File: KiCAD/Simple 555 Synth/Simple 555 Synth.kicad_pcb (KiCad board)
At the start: 2 copper layers, 10 parts, among them P1 PWR_5v, P4 EasyLAB_LOGO, U1 555-timer, U2 555-timer

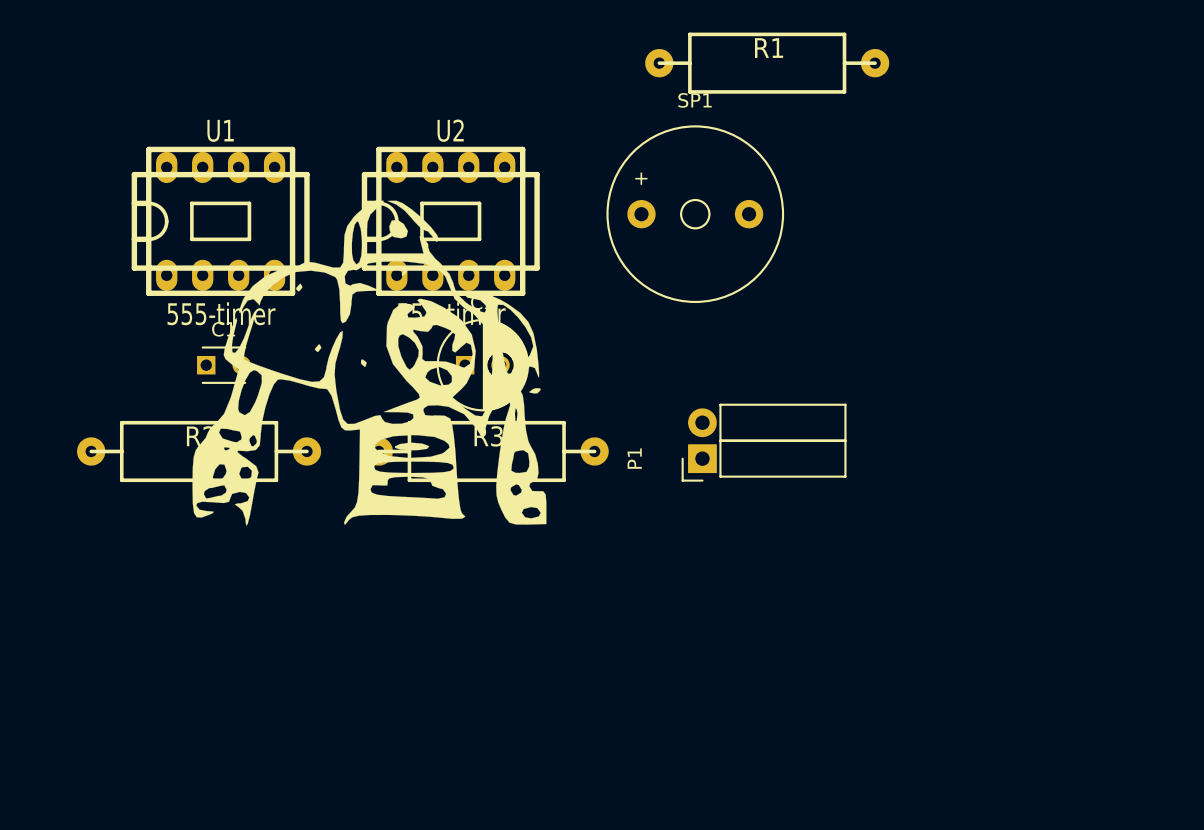
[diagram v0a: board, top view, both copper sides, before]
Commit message: schema en printplaat Versie 20180625 0.6
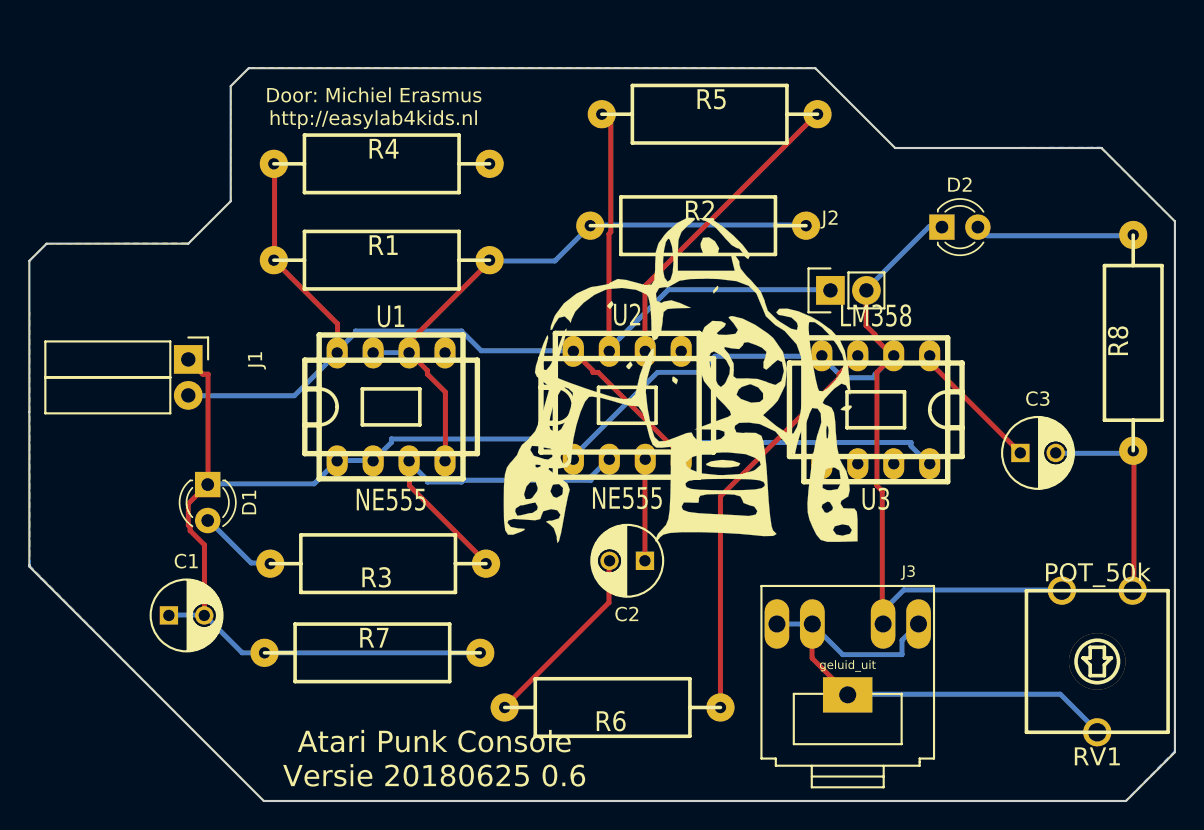
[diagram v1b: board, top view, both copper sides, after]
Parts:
- removed P1: PWR_5v, Socket_Strips:Socket_Strip_Angled_1x02
- removed SP1: Luidspreker, Buzzers_Beepers:Buzzer_12x9.5RM7.6
- added C2: 10uF, Capacitors_ThroughHole:C_Radial_D5_L11_P2.5, F.Cu at (66.5, 53.4)
- added D1: LED1, LEDs:LED_D3.0mm, F.Cu at (35.7, 48.1)
- added D2: LED2, LEDs:LED_D3.0mm, F.Cu at (87.5, 29.9)
- added J1: Stroom, Socket_Strips:Socket_Strip_Angled_1x02, F.Cu at (34.3, 39.2)
- added J2: CapacitorInput, Socket_Strips:Socket_Strip_Straight_1x02, F.Cu at (79.7, 34.3)
- added J3: geluid_uit, footprints:Tayda_3.5mm_stereo_TRS_jack_A-853, F.Cu at (80.9, 61.3)
- added R4: R470K, w_pth_resistors:RC07, F.Cu at (48.0, 25.4)
- added R5: R_PHOTO2, w_pth_resistors:RC07, F.Cu at (71.1, 21.9)
- added R6: R1K, w_pth_resistors:RC07, F.Cu at (64.3, 63.8)
- added R7: R1K, w_pth_resistors:RC07, F.Cu at (47.3, 59.9)
- added R8: R1k, w_pth_resistors:RC07, F.Cu at (101.0, 38.0)
- added RV1: POT_50k, w_pth_resistors:trimmer_ecp_ca9-v10, F.Cu at (98.5, 60.6)
- added U3: LM358, w_pth_circuits:dil_8-300_socket, F.Cu at (82.9, 42.8)
- C1: value 01.uF -> 0.1uF; footprint Capacitors_ThroughHole:C_Disc_D3_P2.5 -> Capacitors_ThroughHole:C_Radial_D5_L11_P2.5
- C3: footprint Capacitors_ThroughHole:C_Radial_D6.3_L11.2_P2.5 -> Capacitors_ThroughHole:C_Radial_D5_L11_P2.5
- R1: value R100k -> R470K
- R2: value R1k -> R_PHOTO1
- R3: value R50k -> R1K
- U1, U2: value 555-timer -> NE555
- moved C3 39.7 mm to (93.1, 45.8)
- moved R2 38.7 mm to (70.3, 29.8)
- moved R1 30.6 mm to (48.0, 32.2)
- moved P4 22.0 mm to (69.1, 40.4)
- moved U2 18.0 mm to (65.3, 42.5)
- moved C1 17.9 mm to (32.9, 57.3)
- moved U1 17.8 mm to (48.6, 42.6)
- moved R3 11.0 mm to (47.7, 53.6), turned to 180 degrees
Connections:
- C1 pad 1: /TRG -> /TRG1
- C1 pad 2: /DIS -> /TRG1
- C3 pad 1: /SPKR -> Net-(C3-Pad1)
- R1 pad 1: /DIS2 -> /RST2
- R1 pad 2: /VSS -> /RST1
- R2 pad 1: /THR -> /RST1
- R2 pad 2: /DIS -> /RST1
- R3 pad 1: /DIS -> /geluid1
- R3 pad 2: /VSS -> Net-(D1-Pad2)
- U1 pad 1: /VSS -> /TRG1
- U1 pad 2: /TRG -> /TRG1
- U1 pad 3: /OUT -> /geluid1
- U1 pad 4: /OUT -> /RST1
- U1 pad 6: /THR -> /RST1
- U1 pad 7: /DIS -> /RST1
- U1 pad 8: /RESET2 -> /RST2
- U2 pad 1: /VSS -> /TRG1
- U2 pad 2: /OUT -> /geluid1
- U2 pad 3: /SPKR -> Net-(C2-Pad1)
- U2 pad 4: /RESET2 -> /RST2
- U2 pad 6: /DIS2 -> Net-(R5-Pad2)
- U2 pad 7: /DIS2 -> /Cap+
- U2 pad 8: /RESET2 -> /RST2
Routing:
- net /TRG1: track 0.00 -> 145.5 mm
- net /RST2: track 0.00 -> 75.2 mm
- net /RST1: track 0.00 -> 43.8 mm
- net Net-(J3-Pad1): track 0.00 -> 37.5 mm
- net /Cap+: track 0.00 -> 34.8 mm
- net Net-(R6-Pad1): track 0.00 -> 28.9 mm
- net /geluid1: track 0.00 -> 25.3 mm
- net Net-(R5-Pad2): track 0.00 -> 21.9 mm
- net Net-(C3-Pad2): track 0.00 -> 15.7 mm
- net Net-(C2-Pad2): track 0.00 -> 13.4 mm
- net Net-(D2-Pad2): track 0.00 -> 11.3 mm
- net Net-(C3-Pad1): track 0.00 -> 9.56 mm
- net Net-(C2-Pad1): track 0.00 -> 7.26 mm
- net Net-(D1-Pad2): track 0.00 -> 5.84 mm
- added copper zone on B.Cu, net (none)
- added copper zone on F.Cu, net (none)
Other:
- board outline added: 80.9 x 51.8 mm
- net class Default: trace_width 0.25 -> 0.35
- board text added: "Atari Punk Console Versie 20180625 0.6"
- board text added: "Door: Michiel Erasmus http://easylab4kids.nl"
